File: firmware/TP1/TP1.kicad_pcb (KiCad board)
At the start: 2 copper layers, 27 parts, among them J1 Conn_02x07_Odd_Even, J2 INPUT, J3 POWER, J4 OUTPUT, U1 BU33SD5WG-TR, U2 STM32L021K4Tx, U3 MCP4801

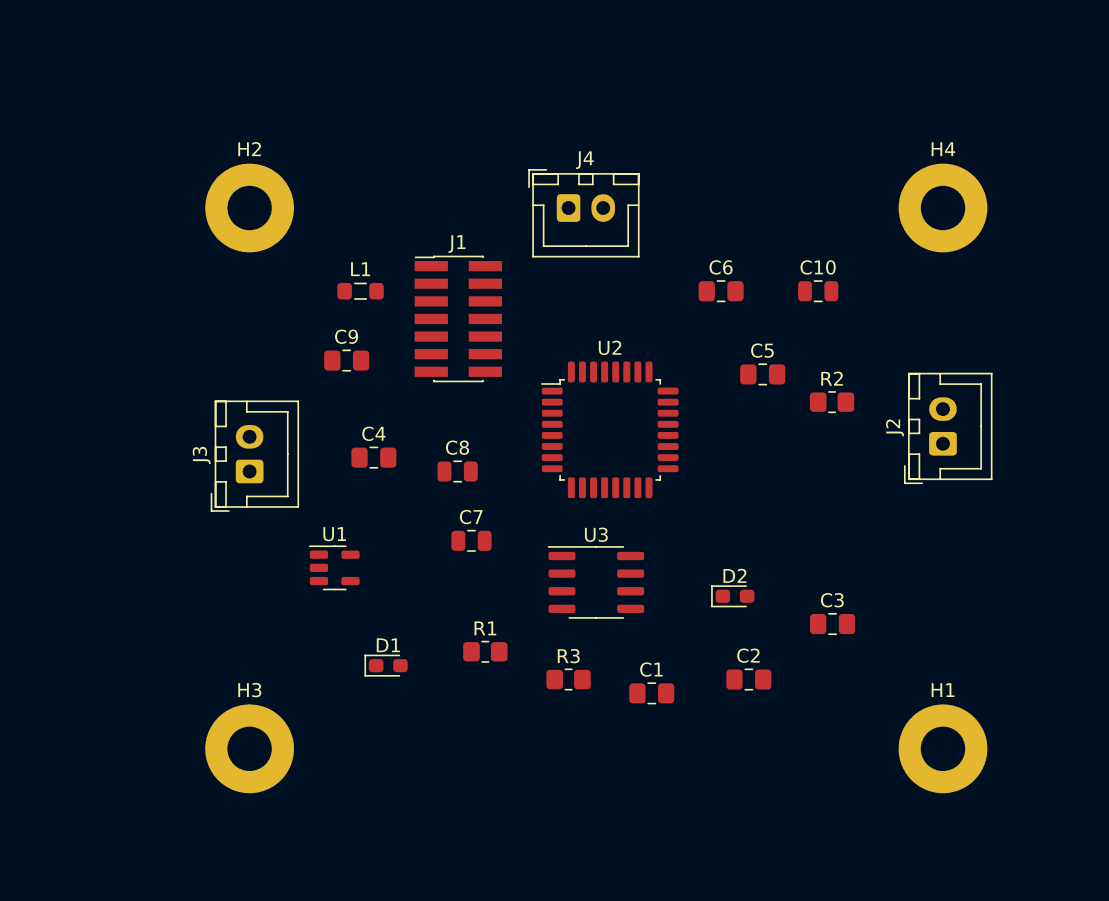
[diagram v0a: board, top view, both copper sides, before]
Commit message: kicad
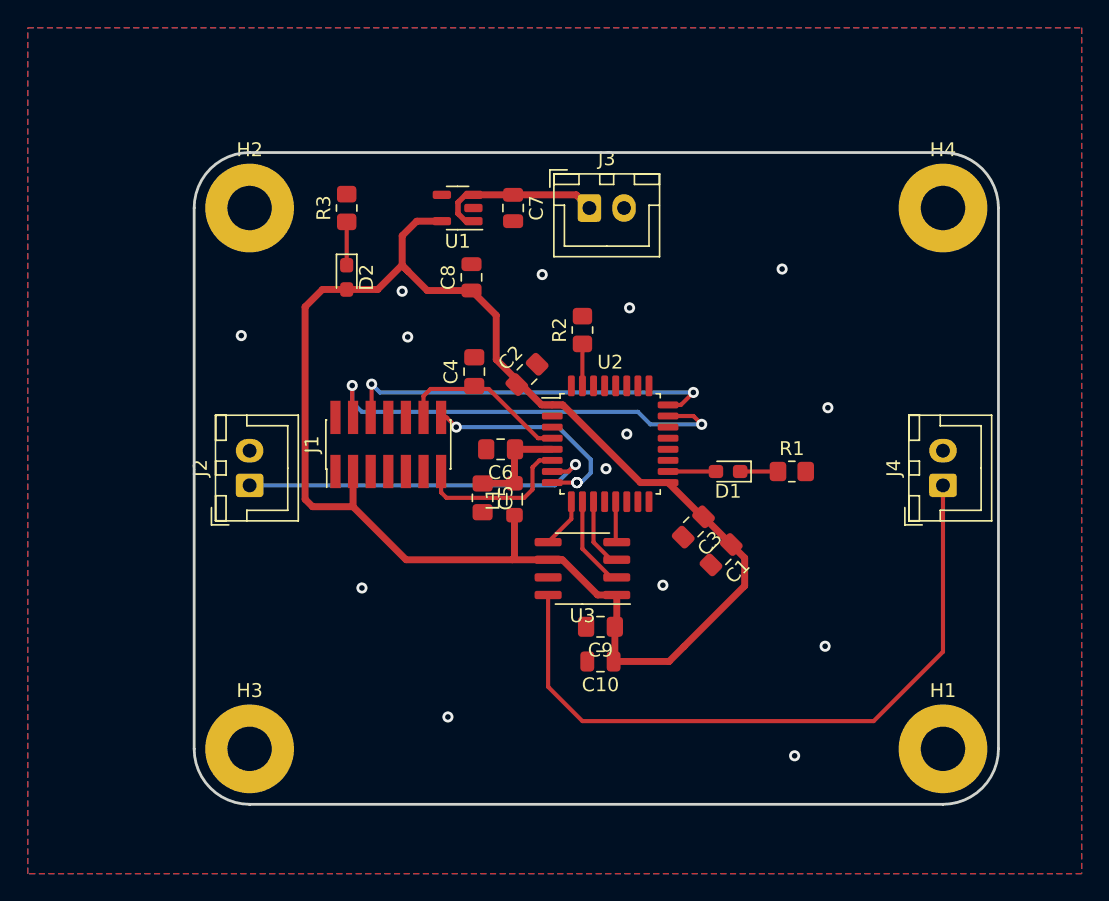
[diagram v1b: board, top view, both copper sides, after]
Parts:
- moved J2 50.1 mm to (64.0, 64.0)
- moved R3 37.6 mm to (71.0, 44.0), turned to 90 degrees
- moved D2 36.2 mm to (71.0, 49.0), turned to -90 degrees
- moved J4 33.6 mm to (114.0, 64.0), turned to 90 degrees
- moved J3 31.0 mm to (88.5, 44.0), turned to 0 degrees
- moved C10 31.0 mm to (89.3, 76.7), turned to 180 degrees
- moved D1 28.2 mm to (98.5, 63.0), turned to 180 degrees
- moved U1 27.4 mm to (79.0, 44.0), turned to 180 degrees
- moved C2 27.2 mm to (84.0, 56.0), turned to 45 degrees
- moved C9 26.5 mm to (89.3, 74.2), turned to 180 degrees
- moved R1 25.6 mm to (103.1, 63.0)
- moved C7 24.2 mm to (83.0, 44.0), turned to -90 degrees
- moved C5 22.1 mm to (80.8, 64.9), turned to -90 degrees
- moved C6 19.6 mm to (82.1, 61.4), turned to 180 degrees
- moved R2 18.7 mm to (88.0, 52.8), turned to 90 degrees
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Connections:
- C5 pad 1: +3.3V -> +3.3VA
- C6 pad 1: +3.3V -> +3.3VA
- L1 pad 2: +3.3V -> +3.3VA
- U2 pad 12: SPI1_MISO -> unconnected-(U2-Pad12)
- U2 pad 18: TIM2_CH1 -> LED_STATUS
- U2 pad 23: SYS_SWDIO -> SWDIO
- U2 pad 24: SYS_SWDCLK -> SWDCK
- U2 pad 7: ADC_ IN1 -> ADC_IN1
- U2 pad 8:  USART2_TX -> USART2_TX
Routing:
- net +3.3V: track 0.00 -> 113.3 mm
- net DAC_OUT: track 0.00 -> 50.2 mm
- net SWDIO: track 0.00 -> 32.1 mm, vias 0 -> 2
- net SWDCK: track 0.00 -> 28.1 mm, vias 0 -> 2
- net ADC_IN1: track 0.00 -> 26.0 mm, vias 0 -> 1
- net USART2_TX: track 0.00 -> 16.1 mm, vias 0 -> 4
- net NRST: track 0.00 -> 12.5 mm
- net +5V: track 0.00 -> 12.2 mm
- net USART2_RX: track 0.00 -> 11.7 mm
- net +3.3VA: track 0.00 -> 7.46 mm
- net DAC_nCS: track 0.00 -> 6.73 mm
- net SPI1_SCK: track 0.00 -> 5.13 mm
- net DAC_nLDAC: track 0.00 -> 3.61 mm
- net LED_STATUS: track 0.00 -> 3.45 mm
- net Net-(D2-Pad1): track 0.00 -> 3.12 mm
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- added copper zone on B.Cu, net GND
- added copper zone on F.Cu, net GND
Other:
- board outline added: 58 x 47 mm
- rule pad_to_mask_clearance: 0 -> 0.1
